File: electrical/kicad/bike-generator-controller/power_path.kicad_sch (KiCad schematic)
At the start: 5 parts, among them J4 PHOENIX 1711725 / RECTIFIER_IN, J5 PHOENIX 1711725 / BUCK_IN

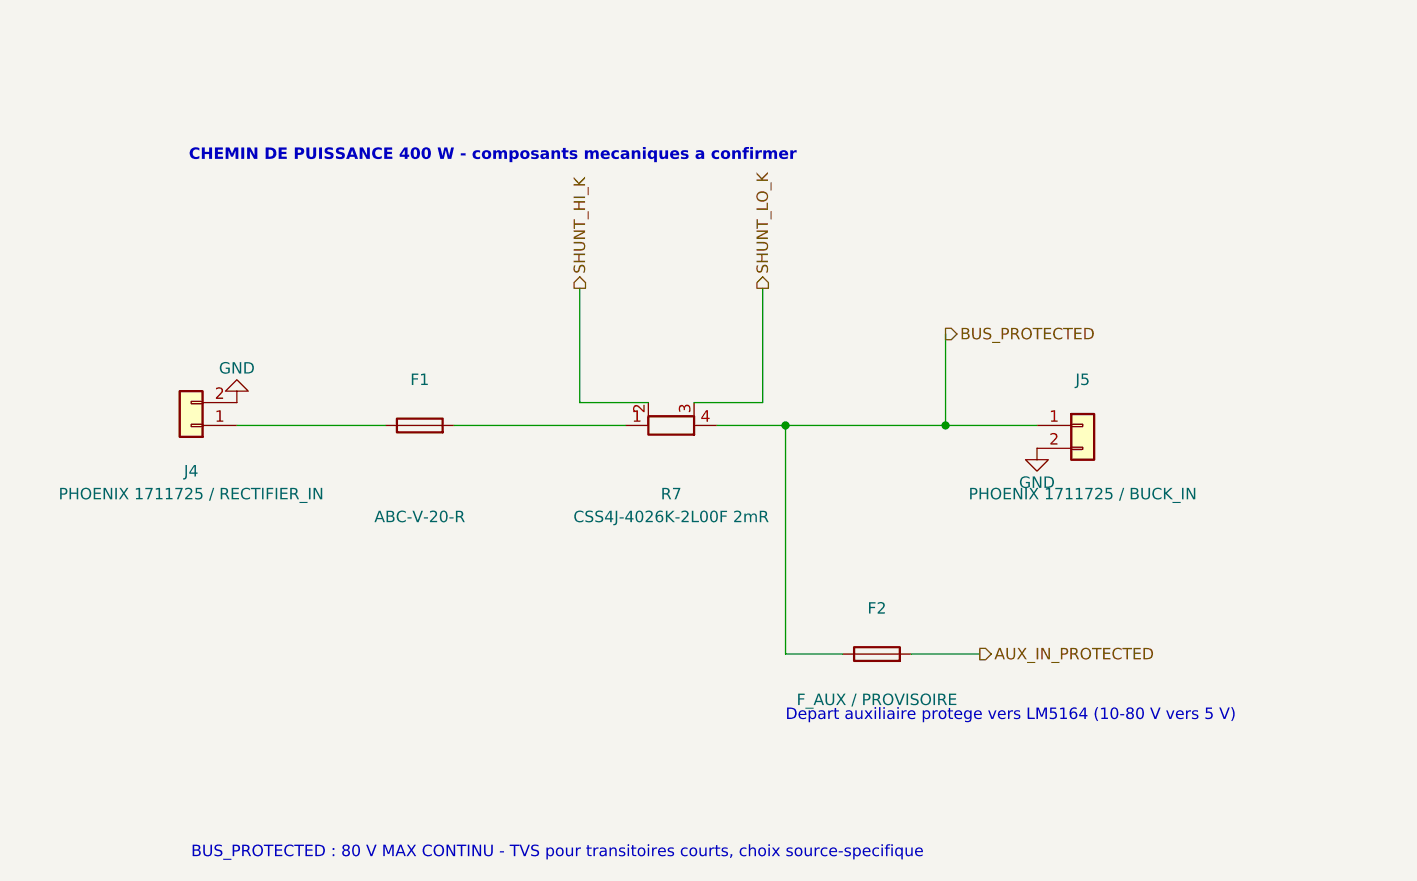
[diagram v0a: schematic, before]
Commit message: wip: checkpoint controller routing before review
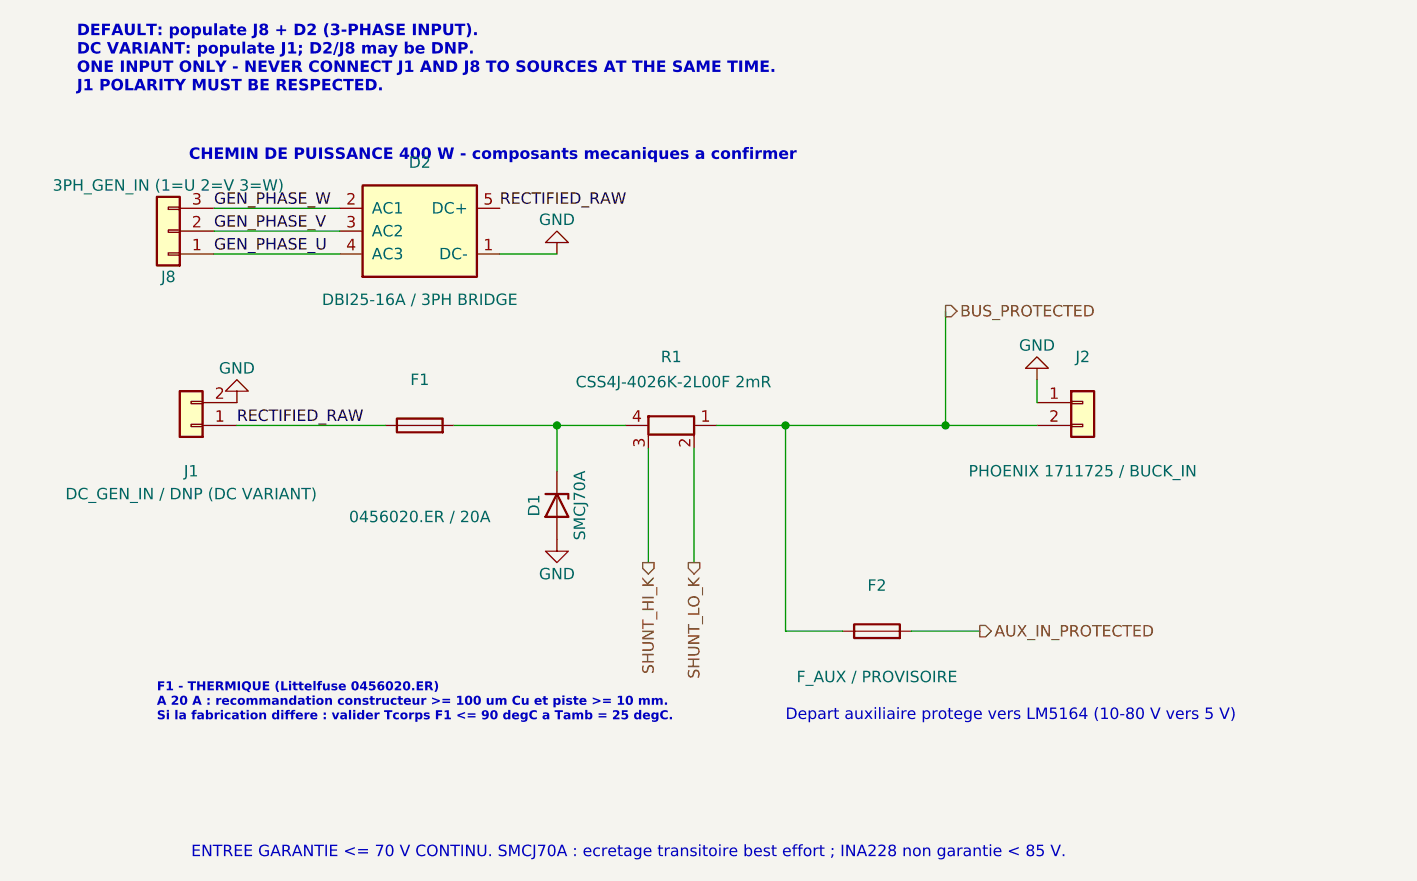
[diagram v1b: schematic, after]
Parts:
- added D1: SMCJ70A, Diode_SMD:D_SMC, symbol Device:D_Zener
- added D2: DBI25-16A / 3PH BRIDGE, BikeGenerator:Diode_Bridge_Diotec_DBI-A_5Pin_P7.50mm, symbol BikeGenerator:DBI25-16A
- added J8: 3PH_GEN_IN (1=U 2=V 3=W), TerminalBlock_Phoenix:TerminalBlock_Phoenix_MKDS-3-3-5.08_1x03_P5.08mm_Horizontal, symbol Connector_Generic:Conn_01x03
- F1: value ABC-V-20-R -> 0456020.ER / 20A; footprint BikeGenerator:Fuse_Eaton_ABC-V-20-R_Axial_P38.10mm -> BikeGenerator:Fuse_Littelfuse_456_10.08x3.05mm_P9.35mm; Interrupt Rating 10 kA at 125 VDC -> 100 A @125 VAC; 300 A @100 VDC; 500 A @72 VDC; 1000 A @32 V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; MPN ABC-V-20-R -> 0456020.ER; Manufacturer Eaton Bussmann -> Littelfuse; Mounting Axial THT -> SMD; Requirement Source-specific; 20A maximum; 125VDC minimum -> 20 A maximum; voltage and interrupt ratings per Littelfuse 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; Thermal_Management (none) -> Rated-current reference: >=100 um copper and >=10 mm trace 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; Voltage Rating 125 VDC / 250 VAC -> 125 VAC / 100 VDC
- J1: renamed from J4; value PHOENIX 1711725 / RECTIFIER_IN -> DC_GEN_IN / DNP (DC VARIANT); Assembly (none) -> DNP by default - DC generator variant only; Warning (none) -> Respect polarity; never use together with J8
- renumbered J5 to J2, R7 to R1
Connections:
- net BUS_PROTECTED: now also J2.2 (Pin_2), R1.1; no longer J2.1 (Pin_1), R1.4
- net GND: now also J2.1 (Pin_1), D1.2 (A), D2.1 (DC-); no longer J2.2 (Pin_2)
- net SHUNT_HI_K: now also R1.3; no longer R1.2
- net SHUNT_LO_K: now also R1.2; no longer R1.3
- net at F1.2: now also R1.4, D1.1 (K); no longer R1.1
- net RECTIFIED_RAW: now reaches F1.1, J1.1 (Pin_1)
- net RECTIFIED_RAW: now also D2.5 (DC+)
- new net GEN_PHASE_U: D2.4 (AC3), J8.1 (Pin_1)
- new net GEN_PHASE_V: D2.3 (AC2), J8.2 (Pin_2)
- new net GEN_PHASE_W: D2.2 (AC1), J8.3 (Pin_3)
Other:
- note added: "DEFAULT: populate J8 + D2 (3-PHASE INPUT). DC VARIANT: populate J1; D2/J8 may be DNP. ONE INPUT ONLY - NEVER CONNECT J1 AND J8 TO SOURCES AT THE SAME TIME. J1 POLARITY MUST BE RESPECTED."
- note added: "ENTREE GARANTIE <= 70 V CONTINU. SMCJ70A : ecretage transitoire best effort ; INA228 non garantie < 85 V."
- note added: "F1 - THERMIQUE (Littelfuse 0456020.ER) A 20 A : recommandation constructeur >= 100 um Cu et piste >= 10 mm. Si la fabrication differe : valider Tcorps F1 <= 90 degC a Tamb = 25 degC."
- note removed: "BUS_PROTECTED : 80 V MAX CONTINU - TVS pour transitoires courts, choix source-specifique"
- moved on the sheet: F2, J2, R1
